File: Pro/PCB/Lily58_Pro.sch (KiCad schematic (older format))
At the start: 85 parts, among them J1 LED, J2 4PIN, J3 OLED, P1 i2c_pin, P2 i2c_pin, SW1 SW_PUSH, SW10 SW_PUSH, SW11 SW_PUSH, SW12 SW_PUSH, SW13 SW_PUSH, SW14 SW_PUSH, SW15 SW_PUSH, SW16 SW_PUSH, SW17 SW_PUSH, SW18 SW_PUSH, SW19 SW_PUSH, SW2 SW_PUSH, SW20 SW_PUSH, SW21 SW_PUSH, SW22 SW_PUSH, SW23 SW_PUSH, SW24 SW_PUSH, SW25 Rotary_Encoder_Switch, SW26 SW_PUSH, SW27 SW_PUSH, SW28 SW_PUSH, SW29 SW_PUSH, SW3 SW_PUSH, SW30 SW_PUSH, SW4 SW_PUSH, SW5 SW_PUSH, SW6 SW_PUSH, SW7 SW_PUSH, SW8 SW_PUSH, SW9 SW_PUSH, U1 ProMicro

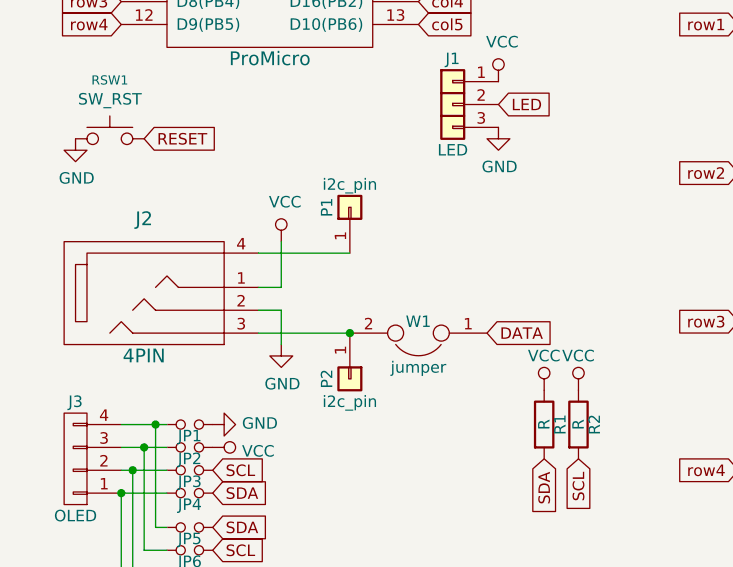
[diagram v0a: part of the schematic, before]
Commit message: Working on routing
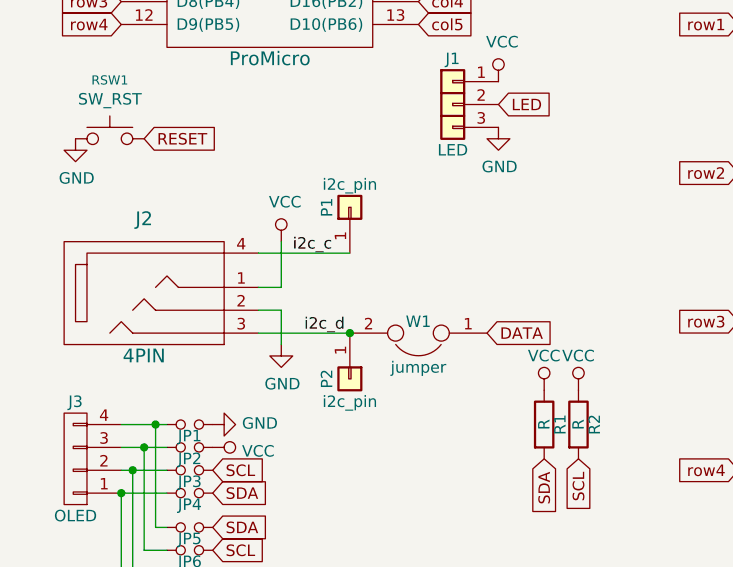
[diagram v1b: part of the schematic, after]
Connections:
- net i2c_d: now reaches J2.3, P2.1 (Pin_1), W1.2
- net i2c_c: now reaches J2.4, P1.1 (Pin_1)
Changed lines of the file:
@@
 Wire Wire Line
 	3400 6150 3400 6250
+Text Label 3350 4550 0    50   ~ 0
+i2c_d
+Text Label 3300 4200 0    50   ~ 0
+i2c_c
 $EndSCHEMATC
